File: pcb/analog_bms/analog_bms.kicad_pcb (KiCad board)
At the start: 2 copper layers, 42 x 22 mm, 51 parts, among them J1 Screw_Terminal_1x2, J2 MODULE+, J3 MODULE-, Q1 PMOS, Q2 NMOS, Q3 PMOS, Q4 NMOS, Q5 PMOS, U1 TLV7031DBV, U2 TLV7031DBV, U3 TLV7032QDDFRQ1, U4 TPS71518DCKRM3, U6 LTC1754

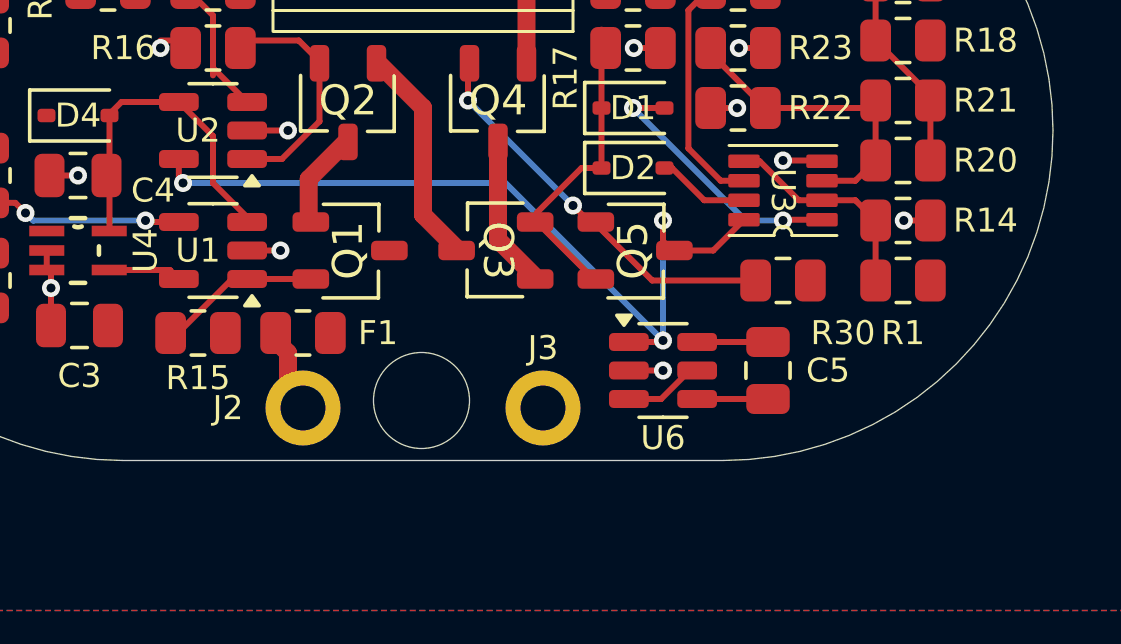
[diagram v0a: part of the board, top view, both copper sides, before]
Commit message: Black PCB + Renders
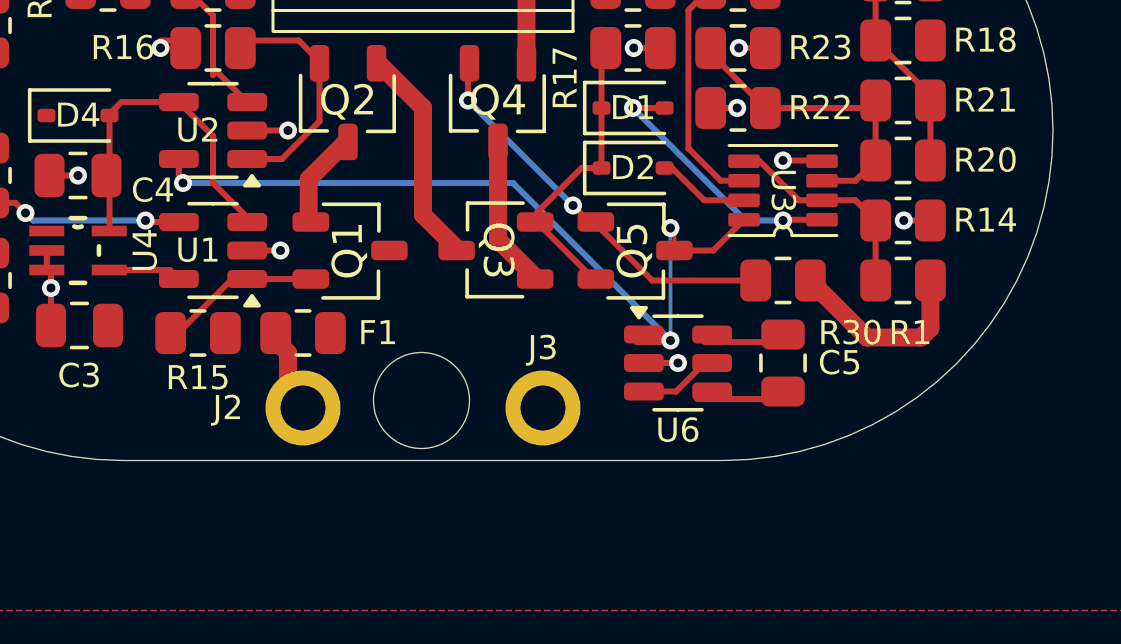
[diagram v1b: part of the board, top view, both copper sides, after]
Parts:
- moved C5 0.56 mm to (151.0, 121.8)
- moved U6 0.56 mm to (147.5, 121.8)
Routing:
- net +BATT: track 5.71 -> 12.2 mm
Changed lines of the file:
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@@
 			(layer "F.Mask"
 				(type "Top Solder Mask")
+				(color "Black")
 				(thickness 0.01)
 			)
@@
 			(layer "B.Mask"
 				(type "Bottom Solder Mask")
+				(color "Black")
 				(thickness 0.01)
 			)
@@
 	(footprint "Capacitor_SMD:C_0805_2012Metric"
 		(layer "F.Cu")
-		(at 150.5 122 -90)
+		(at 151 121.75 -90)
 		(descr "Capacitor SMD 0805 (2012 Metric), square (rectangular) end terminal, IPC-7351 nominal, (Body size source: IPC-SM-782 page 76, https://www.pcb-3d.com/wordpress/wp-content/uploads/ipc-sm-782a_amendment_1_and_2.pdf, https://docs.google.com/spreadsheets/d/1BsfQQcO9C6DZCsRaXUlFlo91Tg2WpOkGARC1WS5S8t0/edit?usp=sharing), generated with kicad-footprint-generator")
 		(tags "capacitor")
 		(property "Reference" "C5"
-			(at 0 -2 180)
+			(at 0 -1.9 180)
 			(layer "F.SilkS")
 			(effects
@@
 		(tags "resistor")
 		(property "Reference" "R1"
-			(at 0 -1.75 0)
+			(at -0.25 -1.75 0)
 			(layer "F.SilkS")
 			(effects
@@
 	(footprint "Package_TO_SOT_SMD:SOT-23-6"
 		(layer "F.Cu")
-		(at 147 122)
+		(at 147.5 121.75)
 		(descr "SOT, 6 Pin (JEDEC MO-178 Var AB https://www.jedec.org/document_search?search_api_views_fulltext=MO-178), generated with kicad-footprint-generator ipc_gullwing_generator.py")
 		(tags "SOT TO_SOT_SMD")
@@
 		(tags "resistor")
 		(property "Reference" "R30"
-			(at 2 1.75 0)
+			(at 2.25 1.75 0)
 			(layer "F.SilkS")
 			(effects
@@
 	)
 	(segment
-		(start 145.8625 122)
-		(end 147 122)
+		(start 146.3625 121.75)
+		(end 147.5 121.75)
 		(width 0.2)
 		(layer "F.Cu")
@@
 	)
 	(via
-		(at 147 122)
+		(at 147.5 121.75)
 		(size 0.6)
 		(drill 0.3)
@@
 	)
 	(segment
-		(start 147.886272 122)
-		(end 148.1375 122)
-		(width 0.2)
+		(start 155.9125 120.5875)
+		(end 155.9125 119)
+		(width 0.6)
 		(layer "F.Cu")
 		(net 2)
@@
 	)
 	(segment
+		(start 153.8 120.9)
+		(end 155.6 120.9)
+		(width 0.6)
+		(layer "F.Cu")
+		(net 2)
+	)
+	(segment
 		(start 128.5414 118.649999)
 		(end 130.562499 118.649999)
@@
 	)
 	(segment
+		(start 155.6 120.9)
+		(end 155.9125 120.5875)
+		(width 0.6)
+		(layer "F.Cu")
+		(net 2)
+	)
+	(segment
+		(start 147.436272 122.7)
+		(end 148.386272 121.75)
+		(width 0.2)
+		(layer "F.Cu")
+		(net 2)
+	)
+	(segment
+		(start 146.3625 122.7)
+		(end 147.436272 122.7)
+		(width 0.2)
+		(layer "F.Cu")
+		(net 2)
+	)
+	(segment
 		(start 150.4125 105)
 		(end 150.4125 104.6625)
@@
 	)
 	(segment
-		(start 146.936272 122.95)
-		(end 147.886272 122)
+		(start 148.386272 121.75)
+		(end 148.6375 121.75)
 		(width 0.2)
 		(layer "F.Cu")
@@
 	)
 	(segment
-		(start 145.8625 122.95)
-		(end 146.936272 122.95)
-		(width 0.2)
+		(start 151.9125 119.0125)
+		(end 153.8 120.9)
+		(width 0.6)
 		(layer "F.Cu")
 		(net 2)
@@
 	)
 	(segment
+		(start 151.9125 119)
+		(end 151.9125 119.0125)
+		(width 0.6)
+		(layer "F.Cu")
+		(net 2)
+	)
+	(segment
 		(start 127.5875 105)
 		(end 127.5875 104.9125)
@@
 	)
 	(segment
-		(start 148.1375 121.05)
-		(end 150.5 121.05)
+		(start 148.3875 121.05)
+		(end 150.75 121.05)
 		(width 0.2)
 		(layer "F.Cu")
@@
 	)
 	(segment
-		(start 146.95 121.05)
-		(end 147 121)
+		(start 147.25 121)
+		(end 147.2 121.05)
 		(width 0.2)
 		(layer "F.Cu")
@@
 	)
 	(segment
-		(start 147 117)
-		(end 147 117.69)
-		(width 0.2)
+		(start 147.38 118)
+		(end 147.31 118)
+		(width 0.127)
 		(layer "F.Cu")
 		(net 15)
 	)
 	(segment
-		(start 147 117.69)
-		(end 147.31 118)
+		(start 147.2 121.05)
+		(end 146.1125 121.05)
 		(width 0.2)
 		(layer "F.Cu")
@@
 	)
 	(segment
-		(start 145.8625 121.05)
-		(end 146.95 121.05)
+		(start 147.38 117.38)
+		(end 147.25 117.25)
+		(width 0.127)
+		(layer "F.Cu")
+		(net 15)
+	)
+	(segment
+		(start 147.31 118)
+		(end 148.675 118)
 		(width 0.2)
 		(layer "F.Cu")
@@
 	)
 	(segment
-		(start 130.8625 114.95)
-		(end 130.8625 115.6125)
+		(start 148.675 118)
+		(end 149.7 116.975)
 		(width 0.2)
 		(layer "F.Cu")
@@
 	)
 	(segment
-		(start 147.31 118)
-		(end 148.675 118)
+		(start 130.8625 114.95)
+		(end 130.8625 115.6125)
 		(width 0.2)
 		(layer "F.Cu")
@@
 	)
 	(segment
-		(start 148.675 118)
-		(end 149.7 116.975)
-		(width 0.2)
+		(start 147.38 118)
+		(end 147.38 117.38)
+		(width 0.127)
 		(layer "F.Cu")
 		(net 15)
 	)
 	(via
-		(at 147 121)
+		(at 147.25 121)
 		(size 0.6)
 		(drill 0.3)
@@
 	)
 	(via
-		(at 131 115.75)
+		(at 147.25 117.25)
 		(size 0.6)
 		(drill 0.3)
@@
 	)
 	(via
-		(at 147 117)
+		(at 131 115.75)
 		(size 0.6)
 		(drill 0.3)
@@
 	)
 	(segment
-		(start 141.75 115.75)
-		(end 147 121)
+		(start 147.25 121)
+		(end 142 115.75)
 		(width 0.2)
 		(layer "B.Cu")
@@
 	)
 	(segment
-		(start 147 121)
-		(end 147 117)
-		(width 0.2)
+		(start 147.25 117.25)
+		(end 147.25 121)
+		(width 0.127)
 		(layer "B.Cu")
 		(net 15)
 	)
 	(segment
-		(start 131 115.75)
-		(end 141.75 115.75)
-		(width 0.2)
-		(layer "B.Cu")
-		(net 15)
-	)
-	(segment
-		(start 147 117)
-		(end 146.972 117.028)
+		(start 142 115.75)
+		(end 131 115.75)
 		(width 0.2)
 		(layer "B.Cu")

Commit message: pepes heh
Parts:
- added G***: LOGO, LOGO, B.Cu at (147.0, 120.7)
- added G***: LOGO, LOGO, B.Cu at (132.0, 109.2)
- added G***: LOGO, LOGO, B.Cu at (125.0, 116.4)
- added G***: LOGO, LOGO, B.Cu at (152.7, 114.8)
